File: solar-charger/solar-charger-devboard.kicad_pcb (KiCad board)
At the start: 2 copper layers, 26.8 x 17 mm, 16 parts, among them IC1 TPS3700DDCR, J1 solar, J2 batt, J3 out, Q1 AO3415, Q2 AO3415

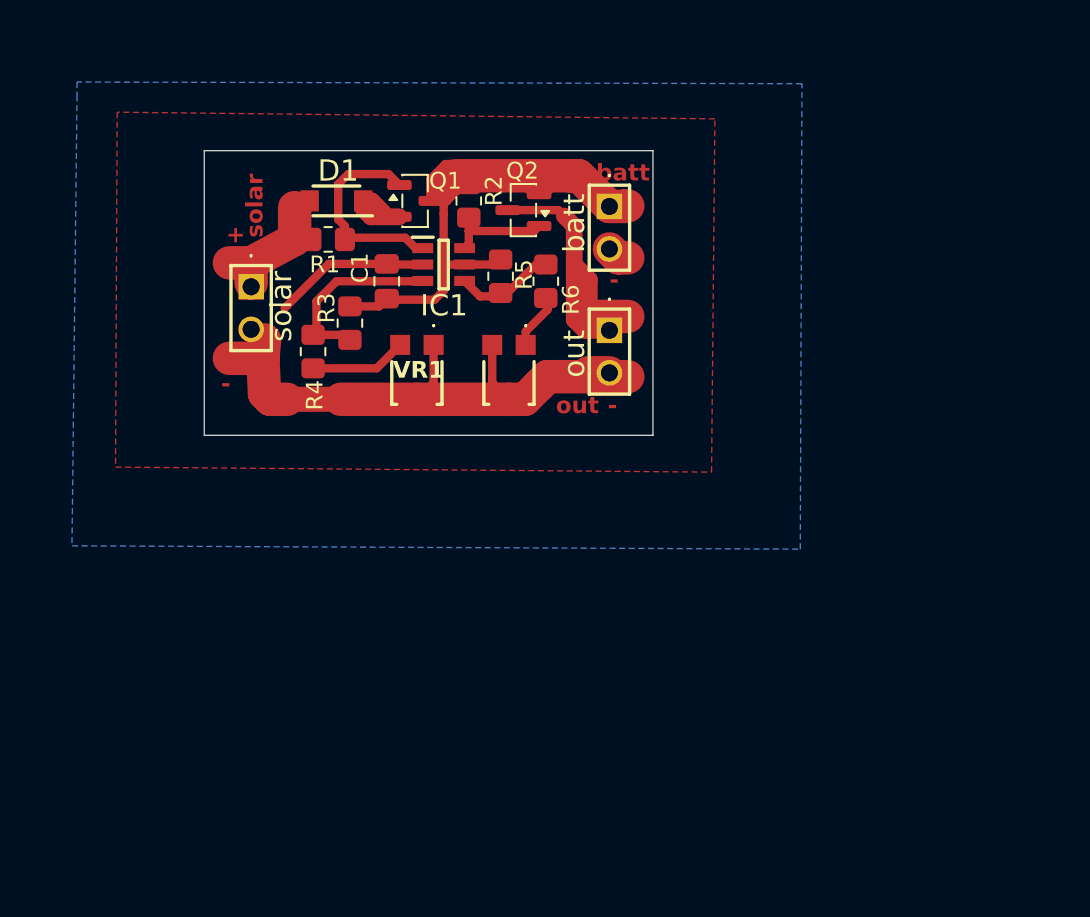
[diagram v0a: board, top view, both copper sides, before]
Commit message: Save
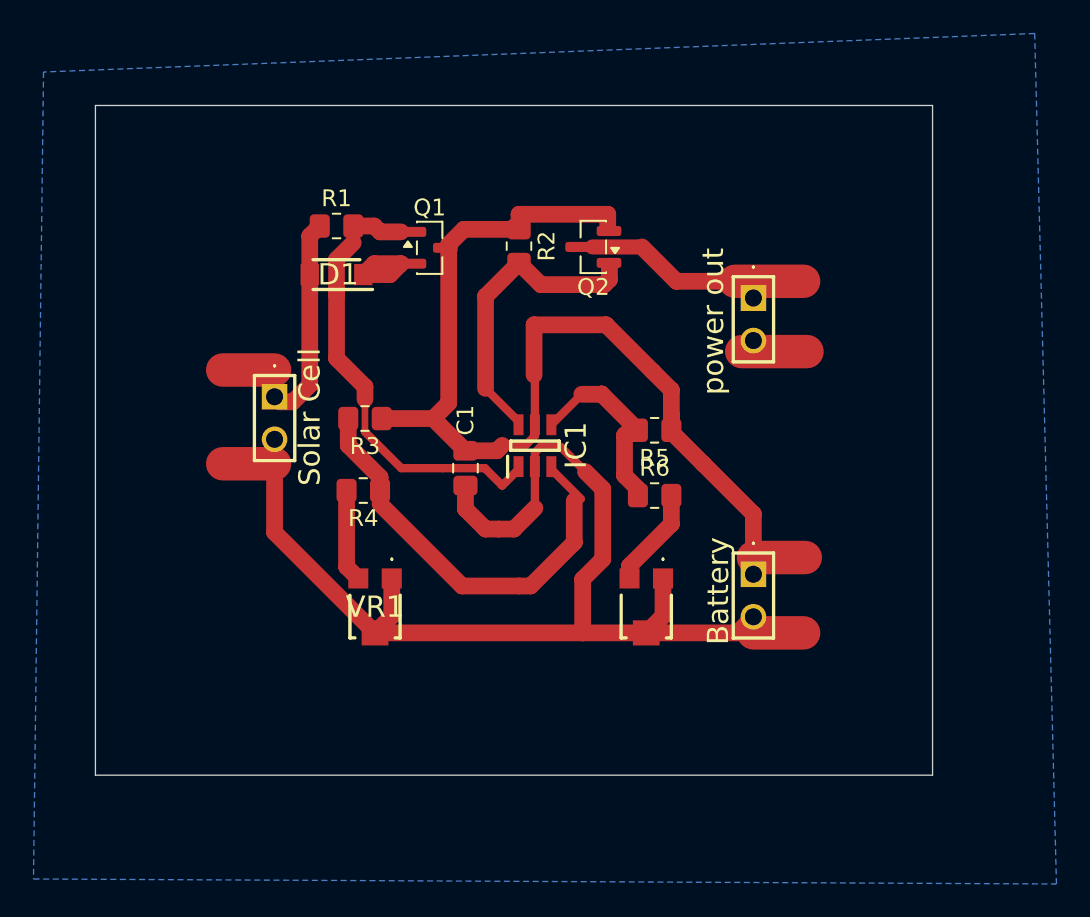
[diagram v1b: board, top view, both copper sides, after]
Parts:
- J1: value solar -> Solar Cell
- J2: value batt -> Battery
- J3: value out -> power out
- moved J2 23.6 mm to (89.1, 78.3)
- moved VR2 16.2 mm to (82.7, 80.3)
- moved R6 14.4 mm to (83.2, 73.6), turned to 0 degrees
- moved VR1 14.2 mm to (66.5, 80.3)
- moved R5 13.0 mm to (83.2, 69.7), turned to 180 degrees
- moved IC1 12.1 mm to (76.0, 70.6), turned to 90 degrees
- moved C1 12.1 mm to (71.9, 72.0), turned to -90 degrees
- moved R4 8.83 mm to (65.8, 73.3), turned to 180 degrees
- moved J3 8.81 mm to (89.1, 61.8)
- moved J1 6.72 mm to (60.5, 67.7)
- moved R3 5.77 mm to (65.9, 69.0), turned to 180 degrees
- moved Q2 4.72 mm to (79.5, 58.8)
- moved D1 4.40 mm to (64.2, 60.4)
- moved R2 4.04 mm to (75.1, 58.7)
- moved Q1 2.93 mm to (69.8, 58.8)
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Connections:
- R6 pad 2: Net-(VR2-CCW) -> Net-(VR2-CW)
- VR2 pad 1: Net-(VR2-CCW) -> -BATT
- VR2 pad 3: -BATT -> Net-(VR2-CW)
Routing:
- net -BATT: track 46.9 -> 82.0 mm
- net +BATT: track 44.2 -> 66.3 mm
- net Net-(IC1-OUTA): track 12.6 -> 28.2 mm
- net Net-(IC1-INA+): track 11.1 -> 25.9 mm
- net Net-(IC1-OUTB): track 6.25 -> 18.2 mm
- net Net-(D1-A): track 8.73 -> 17.1 mm
- net Net-(Q2-D): track 19.9 -> 13.5 mm
- net Net-(VR2-CW): track 0.00 -> 6.14 mm
- net Net-(IC1-INB-): track 6.03 -> 11.7 mm
- net Net-(VR2-CCW): track 3.44 -> 0.00 mm
- net Net-(D1-K): track 3.84 -> 5.04 mm
- removed copper zone on F.Cu, net -BATT
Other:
- board size 26.8 x 17 mm -> 50 x 40 mm
- board text removed: "+"
- board text removed: "-"
- board text removed: "batt"
- board text removed: "out"
- board text removed: "solar"
